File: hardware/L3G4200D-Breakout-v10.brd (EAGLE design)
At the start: 23.5 x 23.5 mm, 14 parts, among them U1 L3G4200D

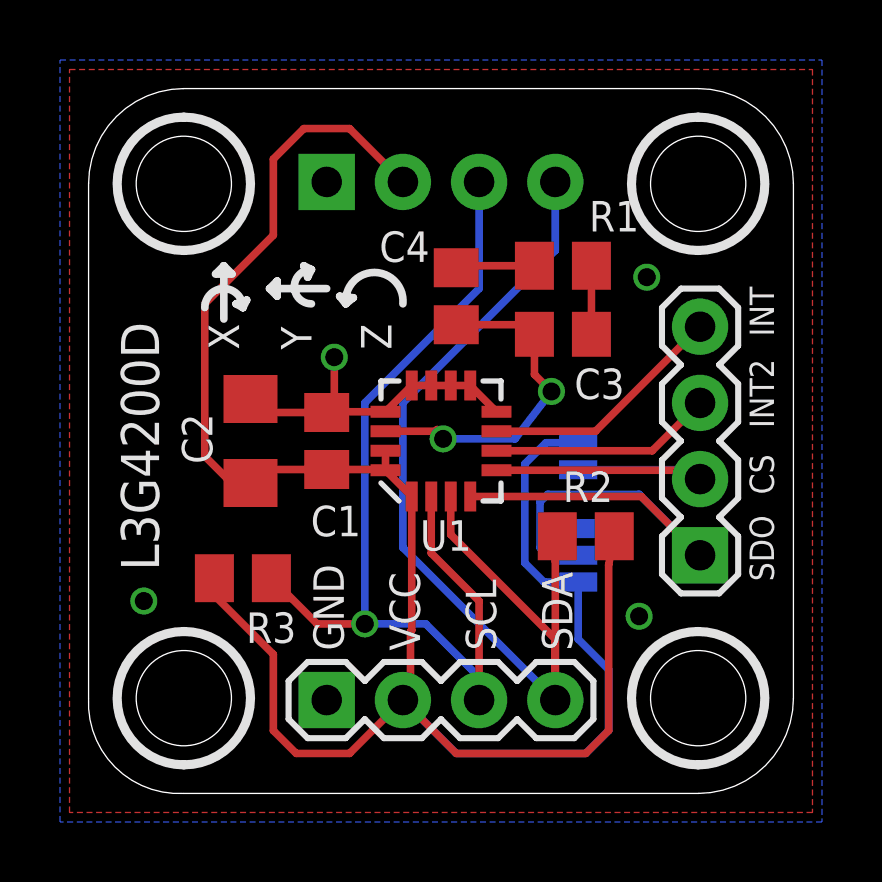
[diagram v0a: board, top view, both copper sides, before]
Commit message: gerbers for Seeedstudio
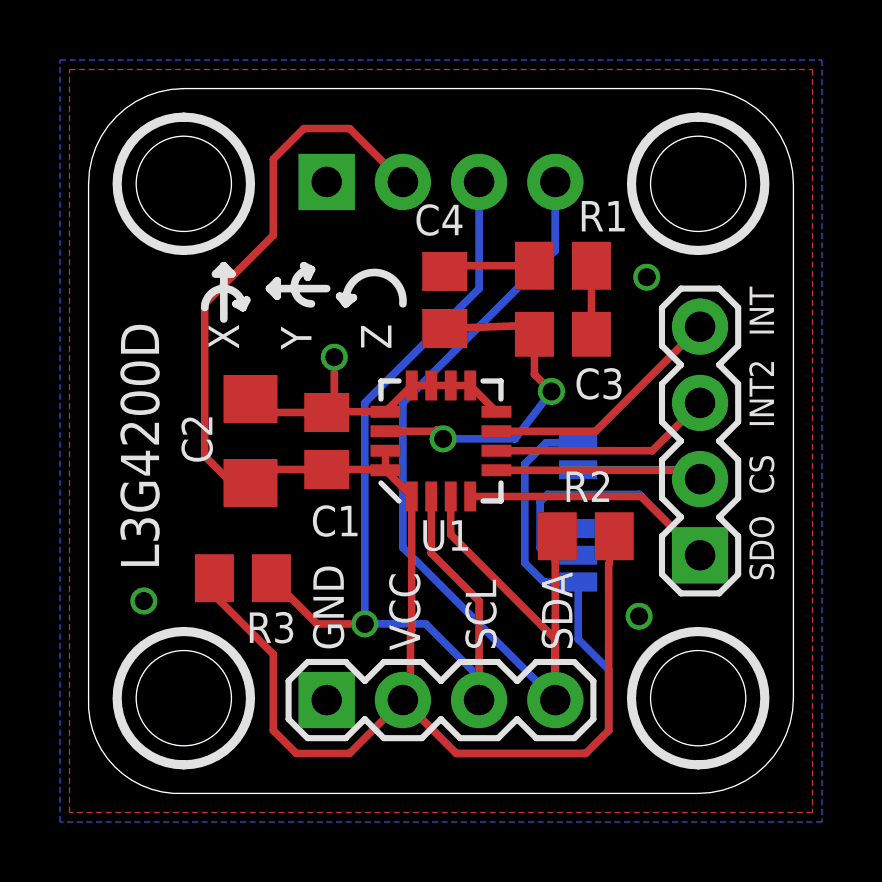
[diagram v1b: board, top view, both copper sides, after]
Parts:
- moved U$3 11.0 mm to (40.1, 15.2), turned to 90 degrees
- moved C4 0.40 mm to (34.2, 17.1)
